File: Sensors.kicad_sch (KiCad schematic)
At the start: 25 parts, among them U19 BME280

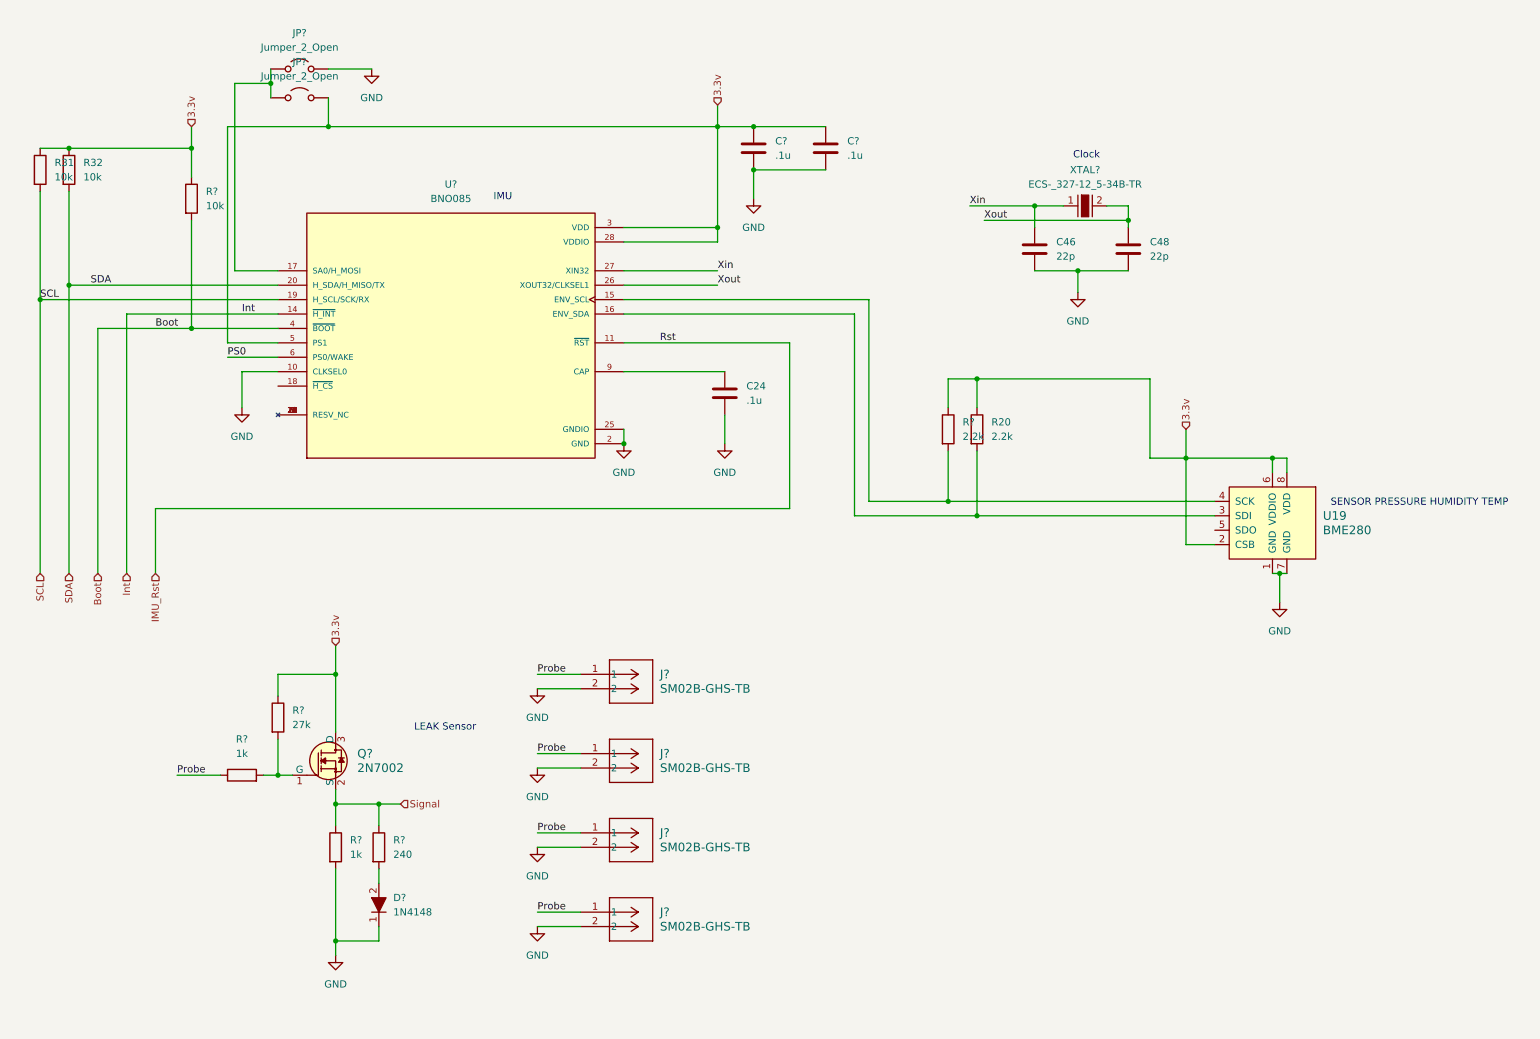
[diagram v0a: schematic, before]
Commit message: stuff
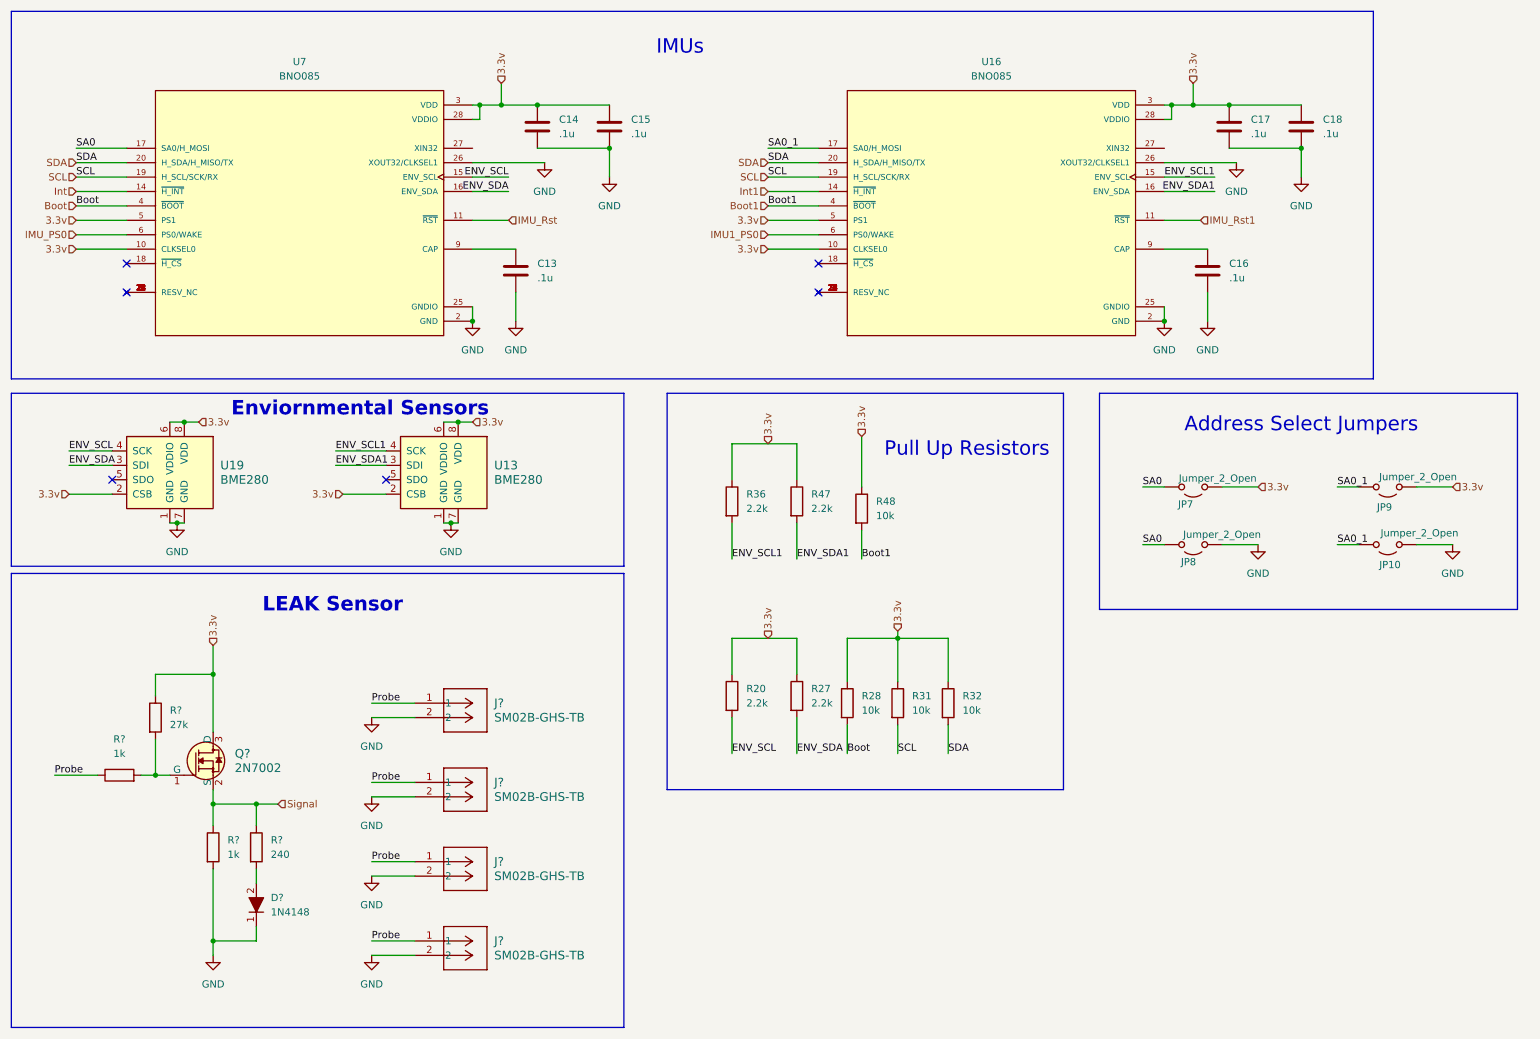
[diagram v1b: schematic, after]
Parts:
- removed C24, C? (x2): .1u, symbol Device:C
- removed C46, C48: 22p, symbol Device:C
- removed JP? (x2): Jumper_2_Open, symbol Jumper:Jumper_2_Open
- removed R?: 10k, symbol Device:R
- removed R?: 2.2k, symbol Device:R
- removed U?: BNO085, BNO085:IC_BNO085, symbol BNO085:BNO085
- removed XTAL?: ECS-_327-12_5-34B-TR, digikey-footprints:SMD-2_3.2x1.5mm, symbol dk_Crystals:ECS-_327-12_5-34B-TR
- added C13, C14, C15, C16, C17, C18: .1u, symbol Device:C
- added JP10, JP7, JP8, JP9: Jumper_2_Open, symbol Jumper:Jumper_2_Open
- added R27, R36, R47: 2.2k, symbol Device:R
- added R28, R48: 10k, symbol Device:R
- added U13: BME280, digikey-footprints:Pressure_Sensor_LGA-8_2.5x2.5mm_BME280, symbol dk_Humidity-Moisture-Sensors:BME280
- added U16, U7: BNO085, BNO085:IC_BNO085, symbol BNO085:BNO085
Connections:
- net 3.3v: now also C14.1, C15.1, C17.1, C18.1, JP7.1 (A), JP9.1 (A), R27.1, R28.1, R36.1, R47.1, R48.1, U13.2 (CSB), U13.6 (VDDIO), U13.8 (VDD), U16.10 (CLKSEL0), U16.28 (VDDIO), U16.3 (VDD), U16.5 (PS1), U7.10 (CLKSEL0), U7.28 (VDDIO), U7.3 (VDD), U7.5 (PS1)
- net Boot: now also R28.2, U7.4 (~{BOOT})
- net GND: now also C13.2, C14.2, C15.2, C16.2, C17.2, C18.2, JP10.1 (A), JP8.1 (A), U13.1 (GND), U13.7 (GND), U16.2 (GND), U16.25 (GNDIO), U16.26 (XOUT32/CLKSEL1), U7.2 (GND), U7.25 (GNDIO), U7.26 (XOUT32/CLKSEL1)
- net IMU_Rst: now also U7.11 (~{RST})
- net Int: now also U7.14 (~{H_INT})
- net SCL: now also U16.19 (H_SCL/SCK/RX), U7.19 (H_SCL/SCK/RX)
- net SDA: now also U16.20 (H_SDA/H_MISO/TX), U7.20 (H_SDA/H_MISO/TX)
- net ENV_SCL: now reaches U19.4 (SCK)
- net ENV_SCL: now also R20.2, U7.15 (ENV_SCL)
- net ENV_SDA: now reaches U19.3 (SDI)
- net ENV_SDA: now also R27.2, U7.16 (ENV_SDA); no longer R20.2
- new net: C13.1, U7.9 (CAP)
- new net: U7.1 (RESV_NC), U7.12 (RESV_NC), U7.13 (RESV_NC), U7.21 (RESV_NC), U7.22 (RESV_NC), U7.23 (RESV_NC), U7.24 (RESV_NC), U7.7 (RESV_NC), U7.8 (RESV_NC)
- new net: U16.1 (RESV_NC), U16.12 (RESV_NC), U16.13 (RESV_NC), U16.21 (RESV_NC), U16.22 (RESV_NC), U16.23 (RESV_NC), U16.24 (RESV_NC), U16.7 (RESV_NC), U16.8 (RESV_NC)
- new net: C16.1, U16.9 (CAP)
- new net Boot1: R48.2, U16.4 (~{BOOT})
- new net ENV_SCL1: R36.2, U13.4 (SCK), U16.15 (ENV_SCL)
- new net ENV_SDA1: R47.2, U13.3 (SDI), U16.16 (ENV_SDA)
- new net IMU1_PS0: U16.6 (PS0/WAKE)
- new net IMU_PS0: U7.6 (PS0/WAKE)
- new net IMU_Rst1: U16.11 (~{RST})
- new net Int1: U16.14 (~{H_INT})
- new net SA0: JP7.2 (B), JP8.2 (B), U7.17 (SA0/H_MOSI)
- new net SA0_1: JP10.2 (B), JP9.2 (B), U16.17 (SA0/H_MOSI)
- no-connect marks 0 -> 6
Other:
- note added: "Address Select Jumpers"
- note added: "Enviornmental Sensors"
- note added: "IMUs"
- note added: "Pull Up Resistors"
- note removed: "Clock"
- note removed: "IMU"
- note removed: "SENSOR PRESSURE HUMIDITY TEMP"
- moved on the sheet: D?, J?, Q?, R?
